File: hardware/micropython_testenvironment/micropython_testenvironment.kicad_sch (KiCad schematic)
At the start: 5 parts, among them J1 RPi_GPIO, J101 USB_B, U101 ESP32-C3-WROOM-02, U102 Pico, U103 Seeed Studio XIAO SAMD21

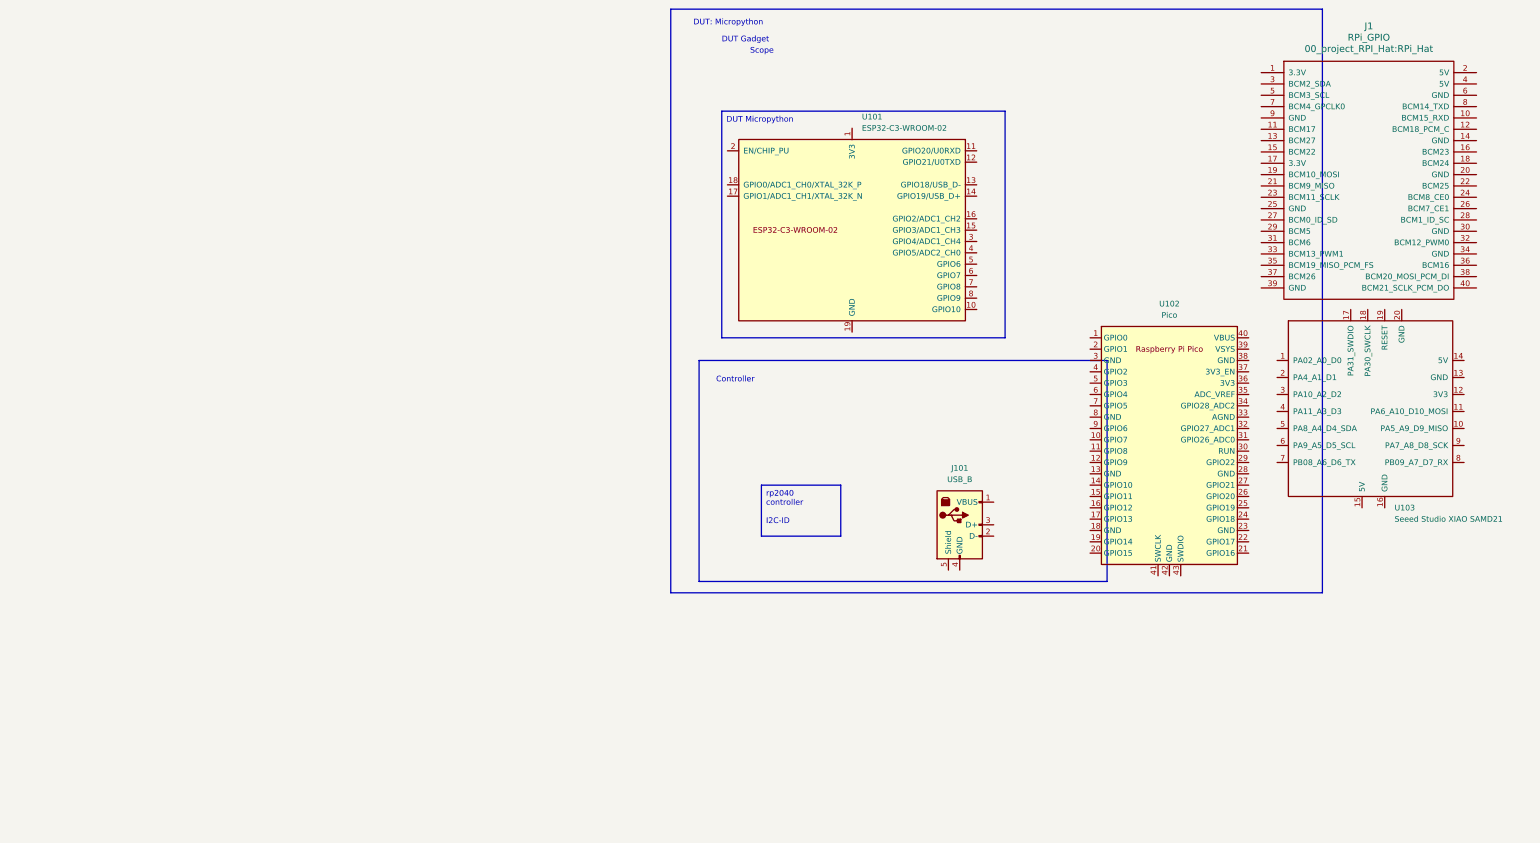
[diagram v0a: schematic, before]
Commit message: Some documentation
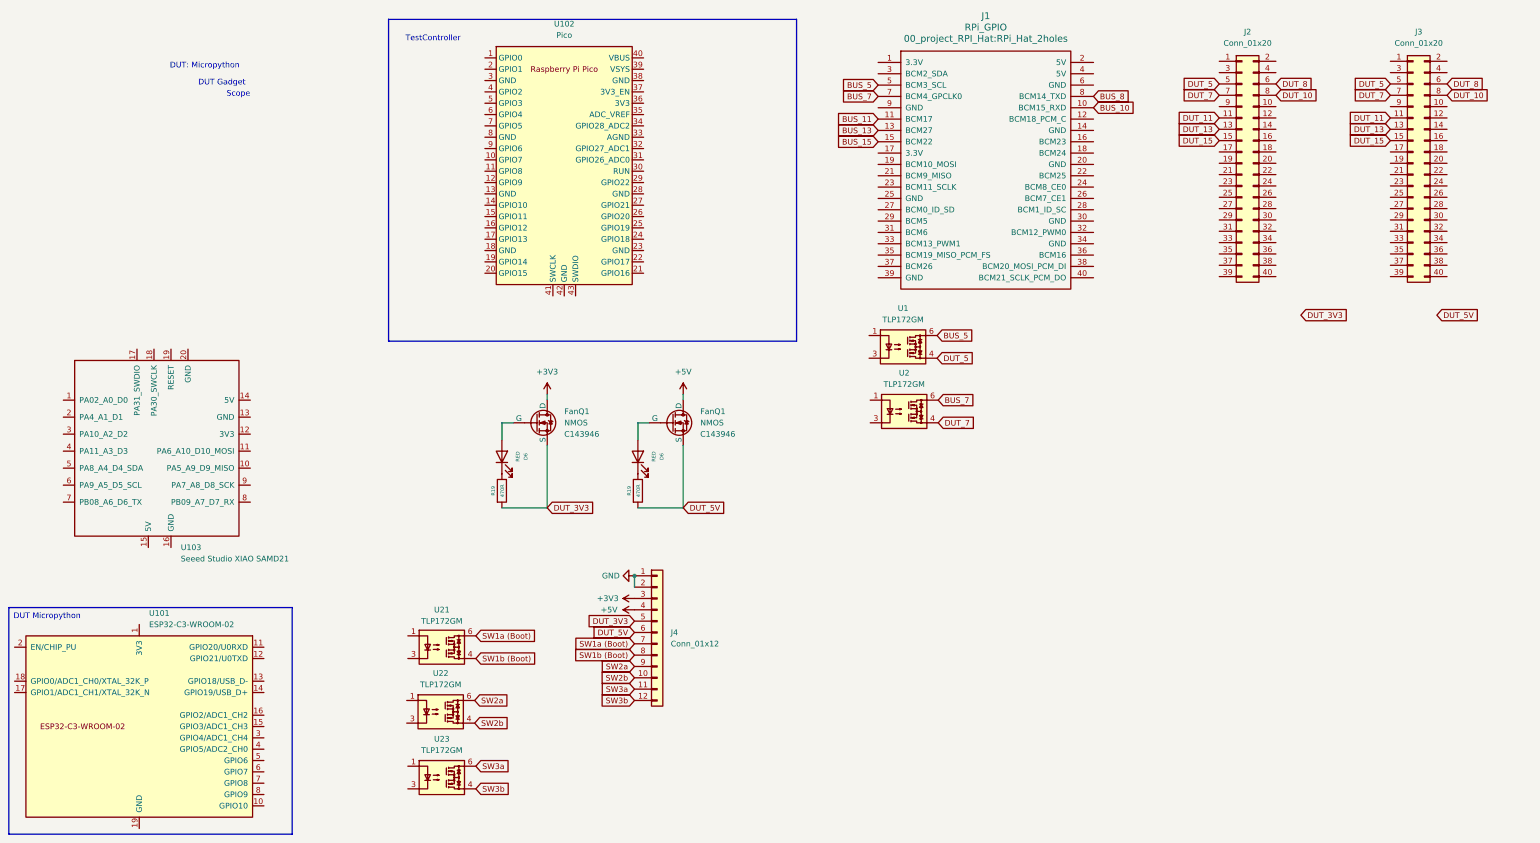
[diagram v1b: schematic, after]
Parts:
- removed J101: USB_B, symbol Connector:USB_B
- added D6 (x2): RED, 00_project_library:LED_0603_1608Metric, symbol 00_project_library:LED
- added FanQ1 (x2): NMOS, 00_project_library:SOT-23, symbol 00_project_library:NMOS
- added J2: Conn_01x20, 00_project_library:PinSocket_2x20_P2.54mm_Vertical-mirrored, symbol Connector_Generic:Conn_02x20_Odd_Even
- added J3: Conn_01x20, 00_project_library:PinSocket_2x20_P2.54mm_Vertical-mirrored-bare, symbol Connector_Generic:Conn_02x20_Odd_Even
- added J4: Conn_01x12, Connector_PinSocket_2.54mm:PinSocket_1x12_P2.54mm_Vertical, symbol Connector_Generic:Conn_01x12
- added R19 (x2): 470R, Resistor_SMD:R_0402_1005Metric_Pad0.72x0.64mm_HandSolder, symbol 00_project_library:R
- added U1, U2, U21, U22, U23: TLP172GM, Package_SO:MFSOP6-4_4.4x3.6mm_P1.27mm, symbol 00_project_library:TLP172GM
- J1: footprint 00_project_RPI_Hat:RPi_Hat -> 00_project_RPI_Hat:RPi_Hat_2holes
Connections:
- net BUS_10: now reaches J1.10 (BCM15_RXD)
- net BUS_11: now reaches J1.11 (BCM17)
- net BUS_13: now reaches J1.13 (BCM27)
- net BUS_15: now reaches J1.15 (BCM22)
- net BUS_5: now reaches J1.5 (BCM3_SCL)
- net BUS_5: now also U1.6
- net BUS_7: now reaches J1.7 (BCM4_GPCLK0)
- net BUS_7: now also U2.6
- net BUS_8: now reaches J1.8 (BCM14_TXD)
- new net: D6.1 (K), R19.1 (x2)
- new net: D6.2 (A), FanQ1.1 (G) (x2)
- new net +3V3: FanQ1.3 (D), J4.3 (Pin_3)
- new net +5V: FanQ1.3 (D), J4.4 (Pin_4)
- new net DUT_10: J2.8 (Pin_8), J3.8 (Pin_8)
- new net DUT_11: J2.11 (Pin_11), J3.11 (Pin_11)
- new net DUT_13: J2.13 (Pin_13), J3.13 (Pin_13)
- new net DUT_15: J2.15 (Pin_15), J3.15 (Pin_15)
- new net DUT_3V3: FanQ1.2 (S), J4.5 (Pin_5), R19.2
- new net DUT_5: J2.5 (Pin_5), J3.5 (Pin_5), U1.4
- new net DUT_5V: FanQ1.2 (S), J4.6 (Pin_6), R19.2
- new net DUT_7: J2.7 (Pin_7), J3.7 (Pin_7), U2.4
- new net DUT_8: J2.6 (Pin_6), J3.6 (Pin_6)
- new net GND: J4.1 (Pin_1), J4.2 (Pin_2)
- new net SW1a (Boot): J4.7 (Pin_7), U21.6
- new net SW1b (Boot): J4.8 (Pin_8), U21.4
- new net SW2a: J4.9 (Pin_9), U22.6
- new net SW2b: J4.10 (Pin_10), U22.4
- new net SW3a: J4.11 (Pin_11), U23.6
- new net SW3b: J4.12 (Pin_12), U23.4
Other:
- note added: "TestController"
- note removed: "Controller"
- moved on the sheet: J1, U101, U102, U103
